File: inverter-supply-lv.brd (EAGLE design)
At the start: 23 x 86.8 mm, 62 parts, among them IC3 1039-2387**3.3V 300mA LDO Vol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, U1 1039-2397** MP2456GJ-Z 0.5A, 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, U2 1039-9015**AOZ1282CI Buck Swi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, X1 0289-9066**15EDGVC-3.81-02P-14

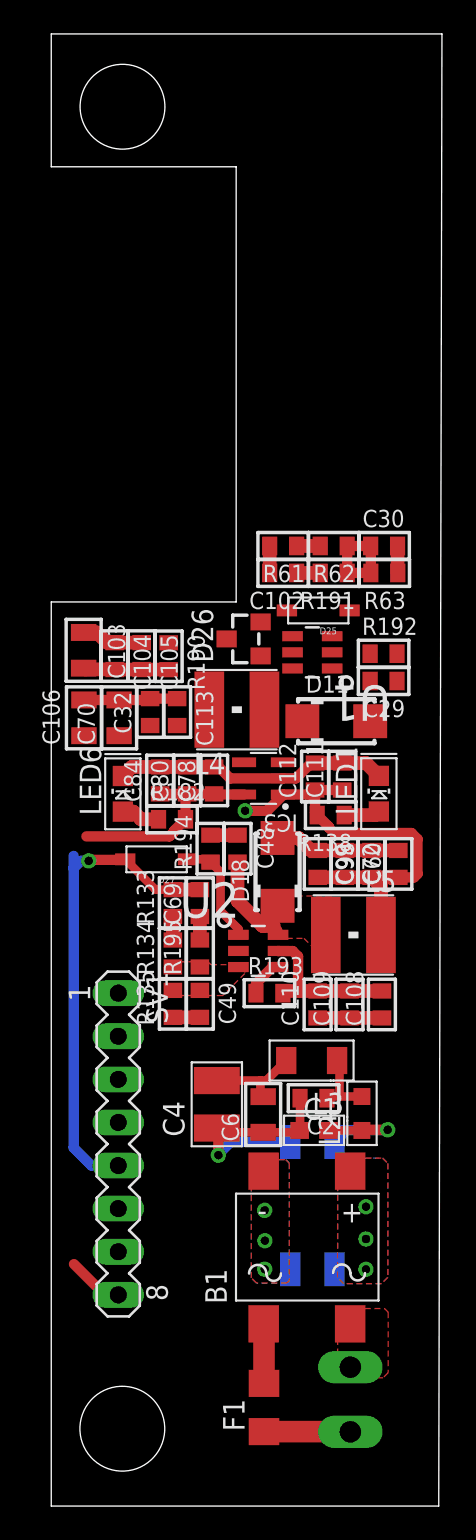
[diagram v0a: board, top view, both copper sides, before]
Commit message: Bitti
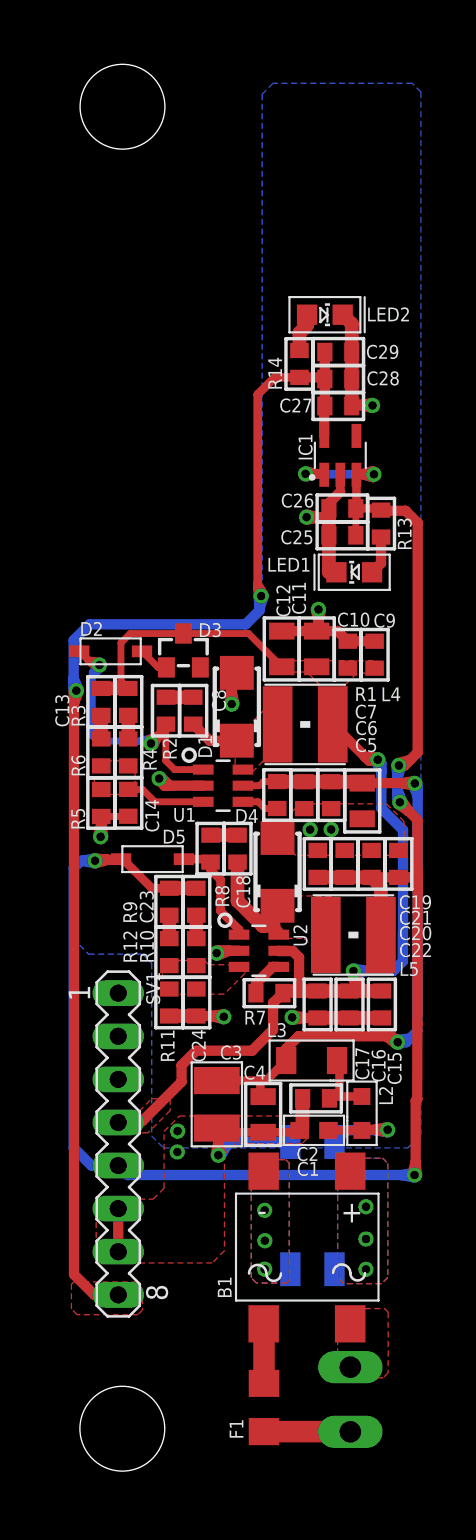
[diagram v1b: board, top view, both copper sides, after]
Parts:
- removed C102, C69: NC, rcl:C0603_ENKO
- removed C103: 4.7uF 50V %10 X7R, rcl:C0805_ENKO
- removed C104, C32: 1200920268**CAP 0603 CER 100nF 50V %10 X7R, rcl:C0603_ENKO
- removed C105, C112, C113, C84: 1200920252**CAP 0603 CER 1nF 50V %10 X7R, rcl:C0603_ENKO
- removed C106, C70: 10uF 50V %10 X7R, rcl:C0805_ENKO
- removed C111, C80: 1019-3166**CAP 0603 CER 100nF 16V %10 X7R (AbC), rcl:C0603_ENKO
- removed C30, C49: 1200920271**CAP 0603 CER 10pF 50V%10 COG, rcl:C0603_ENKO
- removed C78: 1409-0023**CAP 0603 CER 10uf 6.3V %20 X5R, rcl:C0603_ENKO
- removed D11: 1119-3055** DIODE SCHOTTKY 1A 40V DO-214AC SMA DIODES B140-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, diodes:SMA
- removed D25, D27: NC - 1N4148W, adafruit:SOD-123
- removed D26: NC - BZX84CSMD, diode:TO236
- removed IC3: 1039-2387**3.3V 300mA LDO Voltage Regulator TSOP-5, enko:NCP115ASN330T2G
- removed LED6: 1200960006**DIODE LED SMD 0805 RED 10mcd 638nm AlInGaP, led:CHIP-LED0805
- removed R133, R190, R61: 1200970803**RES 0603 100K %1 1/10W, rcl:R0603_ENKO
- removed R134: 1200970584**RES 0603 18K %1 1/10W, rcl:R0603_ENKO
- removed R135: 1200970583**RES 0603 1K %1 1/10W, rcl:R0603_ENKO
- removed R138: 1200970927**RES 0603 100R %1 1/10W, rcl:R0603_ENKO
- removed R182: 1029-2006**RES 0603 47R %1, rcl:R0603_ENKO
- removed R191, R195: NC, rcl:R0603_ENKO
- removed R192: 1200970528**RES 0603 0R %5 1/10W, rcl:R0603_ENKO
- removed R62: 1029-2223**RES 0603 2K4 %1, rcl:R0603_ENKO
- removed R63: 1200970802**RES 0603 3K3 %1 1/10W, rcl:R0603_ENKO
- added C10, C8: 1200920268**CAP 0603 CER 100nF 50V %10 X7R, rcl:C0603_ENKO
- added C11, C12: 10uF 50V %10 X7R, rcl:C0805_ENKO
- added C13, C23: NC, rcl:C0603_ENKO
- added C14, C24: 1200920271**CAP 0603 CER 10pF 50V%10 COG, rcl:C0603_ENKO
- added C25, C28: 1019-3166**CAP 0603 CER 100nF 16V %10 X7R (AbC), rcl:C0603_ENKO
- added C26, C7, C9: 1200920252**CAP 0603 CER 1nF 50V %10 X7R, rcl:C0603_ENKO
- added C27: 1409-0023**CAP 0603 CER 10uf 6.3V %20 X5R, rcl:C0603_ENKO
- added C3: 1019-1016**CAP 1210 CER 10uF 50V %10 X7R (Sadece Murata kul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, ercl:C1210
- added C5: 4.7uF 50V %10 X7R, rcl:C0805_ENKO
- added D1: 1119-3055** DIODE SCHOTTKY 1A 40V DO-214AC SMA DIODES B140-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, diodes:SMA
- added D2, D5: NC - 1N4148W, adafruit:SOD-123
- added D3: NC - BZX84CSMD, diode:TO236
- added IC1: 1039-2387**3.3V 300mA LDO Voltage Regulator TSOP-5, enko:NCP115ASN330T2G
- added LED2: 1200960006**DIODE LED SMD 0805 RED 10mcd 638nm AlInGaP, led:CHIP-LED0805
- added R1, R3, R9: 1200970803**RES 0603 100K %1 1/10W, rcl:R0603_ENKO
- added R10: 1200970584**RES 0603 18K %1 1/10W, rcl:R0603_ENKO
- added R11: 1200970583**RES 0603 1K %1 1/10W, rcl:R0603_ENKO
- added R12, R6: NC, rcl:R0603_ENKO
- added R13: 1200970927**RES 0603 100R %1 1/10W, rcl:R0603_ENKO
- added R14: 1029-2006**RES 0603 47R %1, rcl:R0603_ENKO
- added R2: 1200970528**RES 0603 0R %5 1/10W, rcl:R0603_ENKO
- added R4: 1029-2223**RES 0603 2K4 %1, rcl:R0603_ENKO
- added R5: 1200970802**RES 0603 3K3 %1 1/10W, rcl:R0603_ENKO
- C29: value 1200920268**CAP 0603 CER 100nF 50V %10 X7R -> 1200920252**CAP 0603 CER 1nF 50V %10 X7R
- C4: value 1019-1016**CAP 1210 CER 10uF 50V %10 X7R (Sadece Murata kullanylabilir) -> 10uF 50V %10 X7R; device ercl:C1210 -> rcl:C0805_ENKO
- C6: value 10uF 50V %10 X7R -> 1200920268**CAP 0603 CER 100nF 50V %10 X7R; device rcl:C0805_ENKO -> rcl:C0603_ENKO
- moved C29 19.6 mm to (16.9, 68.0), turned to 0 degrees
- moved C6 19.2 mm to (16.5, 41.9)
- moved LED1 13.1 mm to (17.9, 55.0), turned to 90 degrees
- moved U1 9.46 mm to (10.1, 42.5), turned to 0 degrees
- moved L4 4.12 mm to (15.0, 46.1), turned to 180 degrees
- moved C4 2.80 mm to (12.5, 23.1)
- moved C2 0.15 mm to (15.6, 24.0)
- renumbered C108 to C15, C109 to C16, C110 to C17, C48 to C18, C60 to C20, C72 to C22, C98 to C19, C99 to C21, D18 to D4, R193 to R7, R194 to R8
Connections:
- net +3V3: now also C27.1, C28.1, C29.1, IC1.5, R14.2; no longer C78.1, C80.1, C84.1, IC3.5, R182.2
- net +5V: now also C23.2, C25.1, C26.1, D5.A, IC1.1, IC1.3, R13.2, R9.2; no longer C111.1, C112.1, C69.2, D27.A, IC3.1, IC3.3, R133.2, R138.2
- net DGND: now also C10.1, C11.1, C12.1, C14.2, C24.2, C25.2, C26.2, C27.2, C28.2, C29.2, C3.1, C5.1, C7.1, C9.2, D1.A, IC1.2, LED2.C, R11.1, R5.1; no longer C103.1, C104.1, C105.1, C106.1, C111.2, C112.2, C113.2, C30.2, C32.1, C49.2, C70.1, C78.2, C80.2, C84.2, D11.A, IC3.2, LED6.C, R135.1, R63.1
- net N$1: now also R13.1; no longer R138.1
- net N$105: now also LED2.A, R14.1; no longer LED6.A, R182.1
- net N$11: now also C8.2, D1.C; no longer C29.2, D11.C
- net N$148: now also R1.1; no longer R190.1
- net N$149: now also R3.1, R4.2; no longer R61.1, R62.2
- net N$151: now also D2.C, R2.1; no longer D25.C, R192.1
- net N$152: now also C13.1, R6.2; no longer C102.1, R191.2
- net N$154: now also D2.A, D3.A; no longer D25.A, D26.A
- net N$155: now also R10.2, R9.1; no longer R133.1, R134.2
- net N$159: now also C23.1, R12.2; no longer C69.1, R195.2
- net N$35: now also C8.1, R2.2; no longer C29.1, R192.2
- net N$62: now also D5.C; no longer D27.C
- net N$72: now also C3.2, C5.2, C7.2, R1.2; no longer C103.2, C104.2, C105.2, R190.2
- net VDD: now also C10.2, C11.2, C12.2, C13.2, C9.1, D3.C, R3.2; no longer C102.2, C106.2, C113.1, C32.2, C70.2, D26.C, R61.2
- net V_FB1: now also C14.1, R4.1, R5.2, R6.1; no longer C30.1, R191.1, R62.1, R63.2
- net V_FB2: now also C24.1, R10.1, R11.2, R12.1; no longer C49.1, R134.1, R135.2, R195.1
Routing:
- net N$3: track 0.00 -> 86.8 mm
- net +5V: track 54.6 -> 130.7 mm, vias 2 -> 6
- net +3V3: track 16.6 -> 82.2 mm, vias 0 -> 2
- net N$9: track 0.00 -> 53.3 mm
- net VDD: track 17.1 -> 67.3 mm, vias 0 -> 2
- net N$72: track 10.7 -> 46.8 mm, vias 0 -> 2
- net DGND: track 47.3 -> 74.8 mm, vias 1 -> 14
- net N$7: track 0.00 -> 25.6 mm
- net N$151: track 0.00 -> 23.1 mm, vias 0 -> 2
- net N$2: track 0.00 -> 23.0 mm
- net N$10: track 0.00 -> 23.0 mm
- net N$8: track 0.00 -> 10.9 mm
- net N$5: track 0.00 -> 10.9 mm
- net N$4: track 0.00 -> 7.83 mm
- net N$99: track 6.93 -> 10.5 mm
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- added copper zone on layer 1, net +3V3
- added copper zone on layer 1, net DGND
- added copper zone on layer 16, net DGND
- added copper zone on layer 1, net N$11
- added copper zone on layer 1, net VDD
- added copper zone on layer 1, net V_FB1
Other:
- board outline removed
